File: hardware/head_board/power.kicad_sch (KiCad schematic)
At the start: 11 parts, among them U1 P78E05-1000, U2 MIC5317-3.3

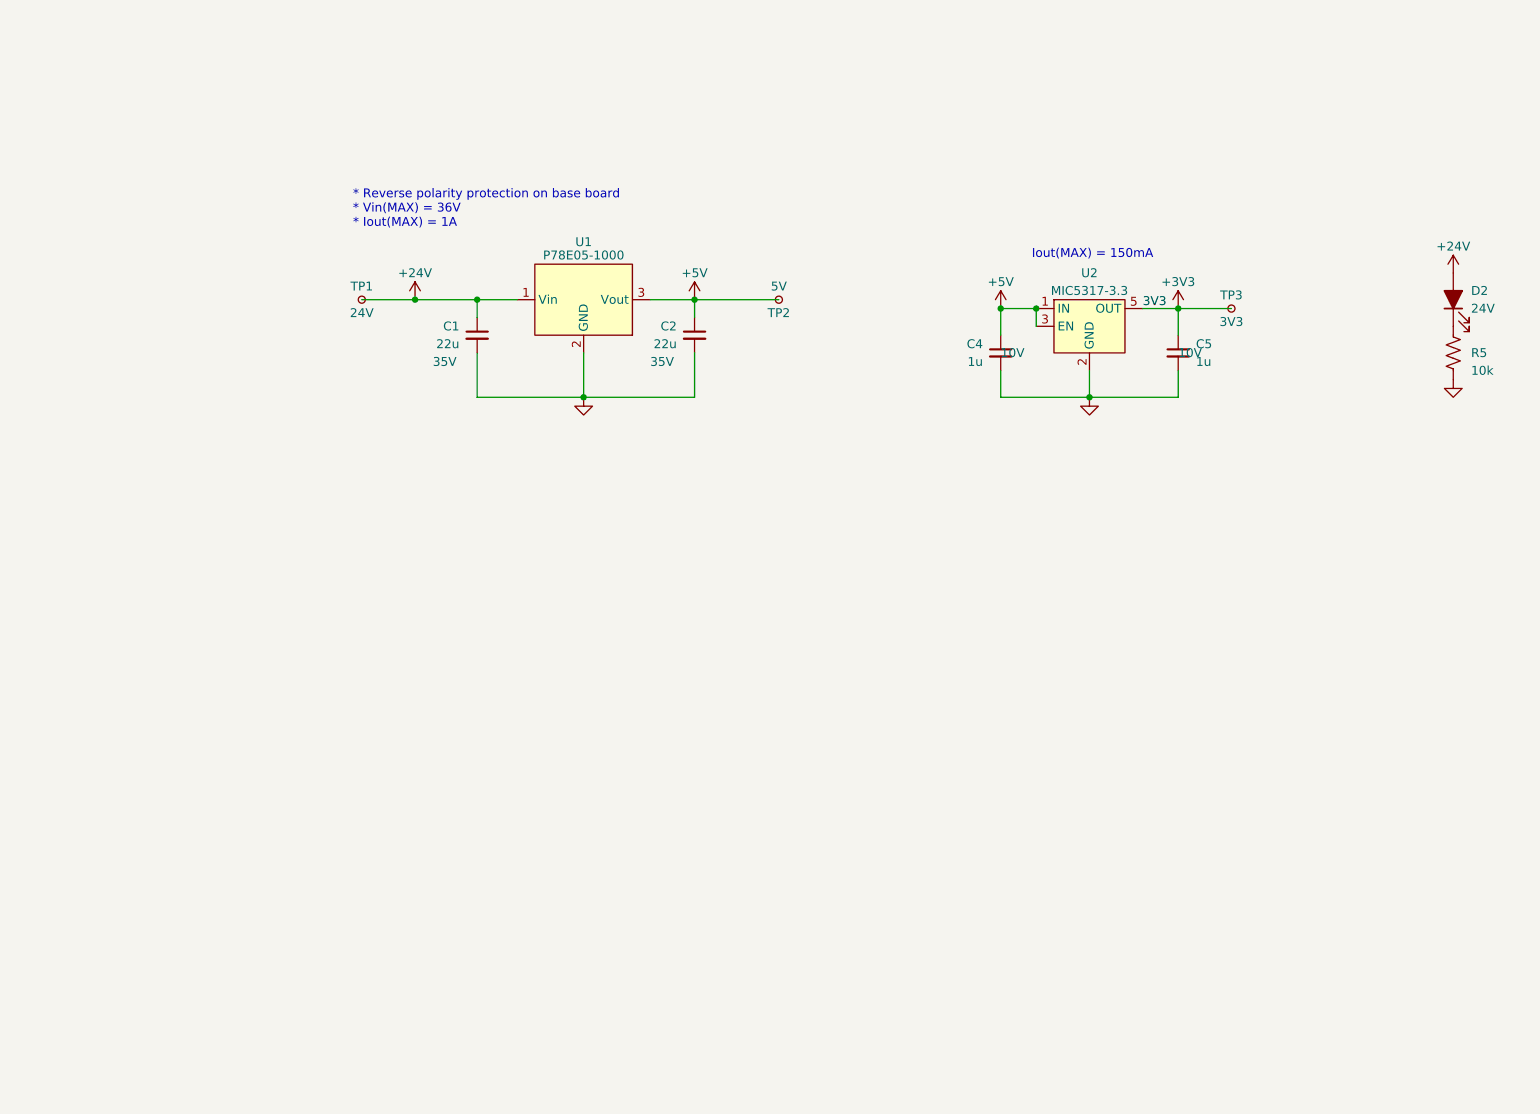
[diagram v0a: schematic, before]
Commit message: v1 revision to the schematic
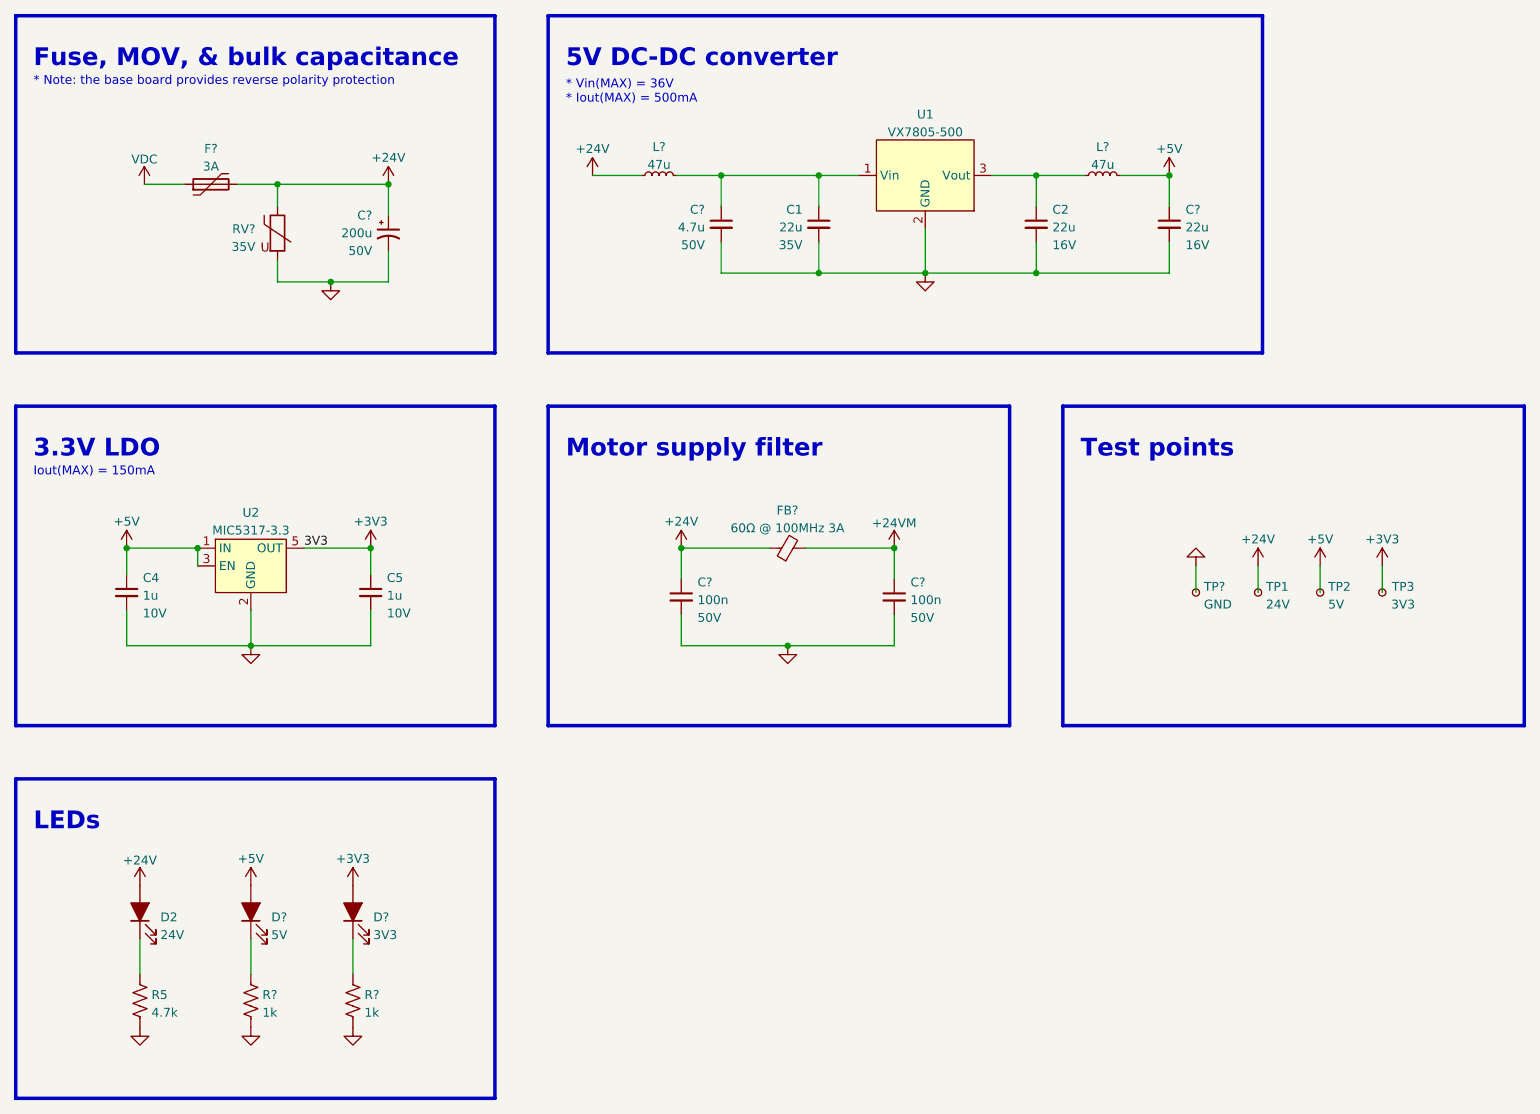
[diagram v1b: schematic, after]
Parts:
- removed U1: P78E05-1000, winterbloom:Converter_DCDC_CUI_P78E-1000_THT, symbol winterbloom:P78E-1000
- added C?: 22u, Capacitor_SMD:C_0805_2012Metric_Pad1.18x1.45mm_HandSolder, symbol Device:C_Small
- added C? (x2): 100n, Capacitor_SMD:C_0402_1005Metric_Pad0.74x0.62mm_HandSolder, symbol Device:C_Small
- added C?: 4.7u, Capacitor_SMD:C_0805_2012Metric_Pad1.18x1.45mm_HandSolder, symbol Device:C_Small
- added C?: 200u, symbol Device:C_Polarized_Small_US
- added D?: 5V, winterbloom:LED_0805_Kingbright_APT2012, symbol Device:LED_Filled
- added D?: 3V3, winterbloom:LED_0805_Kingbright_APT2012, symbol Device:LED_Filled
- added F?: 3A, symbol Device:Polyfuse
- added FB?: 60Ω @ 100MHz 3A, symbol Device:FerriteBead_Small
- added L? (x2): 47u, symbol Device:L_Small
- added R? (x2): 1k, Resistor_SMD:R_0603_1608Metric_Pad0.98x0.95mm_HandSolder, symbol Device:R_US
- added RV?: 35V, symbol Device:Varistor
- added TP?: GND, TestPoint:TestPoint_Pad_1.0x1.0mm, symbol Connector:TestPoint_Small
- added U1: VX7805-500, symbol winterbloom:VX7805-500
- C2: Rating 35V -> 16V
- R5: value 10k -> 4.7k
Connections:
- net +24V: now also C?.1, C?.1, C?.1, F?.2, FB?.1, FB?.2, L?.1, RV?.1; no longer C1.1
- net +3V3: now also D?.2 (A)
- net +5V: now also C?.1, D?.2 (A), L?.2; no longer C2.1
- net GND: now also C?.2, C?.2, C?.2, C?.2, C?.2, R?.2, R?.2, RV?.2, TP?.1, U1.2 (GND)
- new net: C2.1, L?.1, U1.3 (Vout)
- new net: D?.1 (K), R?.1 (x2)
- new net: C1.1, C?.1, L?.2, U1.1 (Vin)
- new net VDC: F?.1
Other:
- note added: "* Note: the base board provides reverse polarity protection"
- note added: "* Vin(MAX) = 36V * Iout(MAX) = 500mA"
- note added: "3.3V LDO"
- note added: "5V DC-DC converter"
- note added: "Fuse, MOV, & bulk capacitance"
- note added: "LEDs"
- note added: "Motor supply filter"
- note added: "Test points"
- note removed: "* Reverse polarity protection on base board * Vin(MAX) = 36V * Iout(MAX) = 1A"
- company: (none) -> Winterbloom
- title: (none) -> Candela Head
- moved on the sheet: C1, C2, C4, C5, D2, R5, TP1, TP2, TP3, U2
